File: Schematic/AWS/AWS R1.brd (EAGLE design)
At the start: 50 x 70 mm, 24 parts, among them U1 SN754410_NE_16

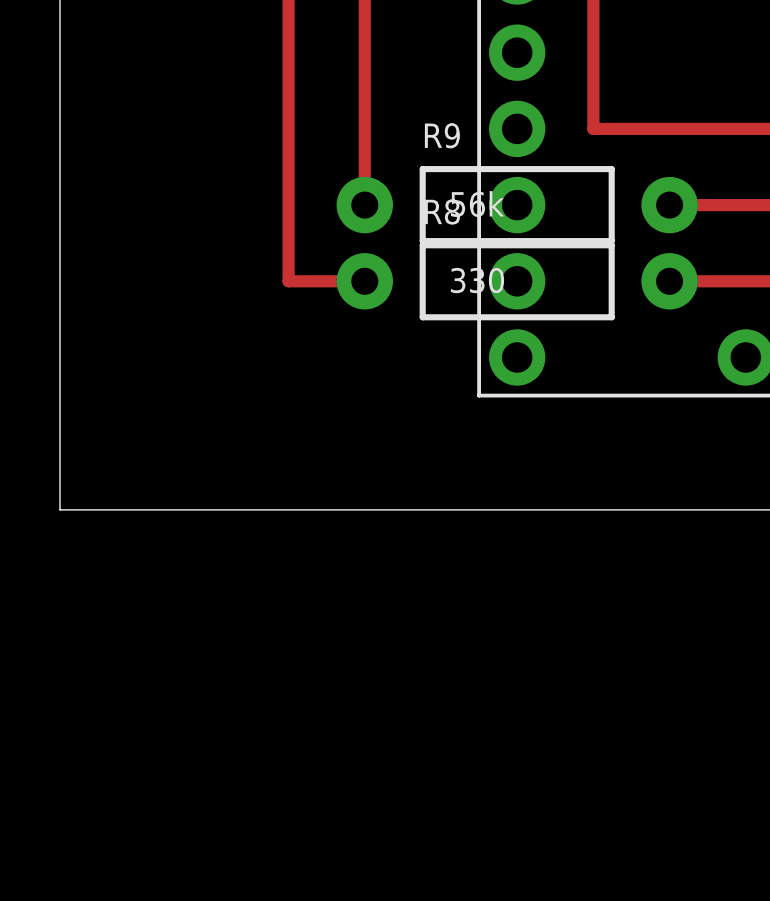
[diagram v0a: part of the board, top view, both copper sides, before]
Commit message: Moved outside
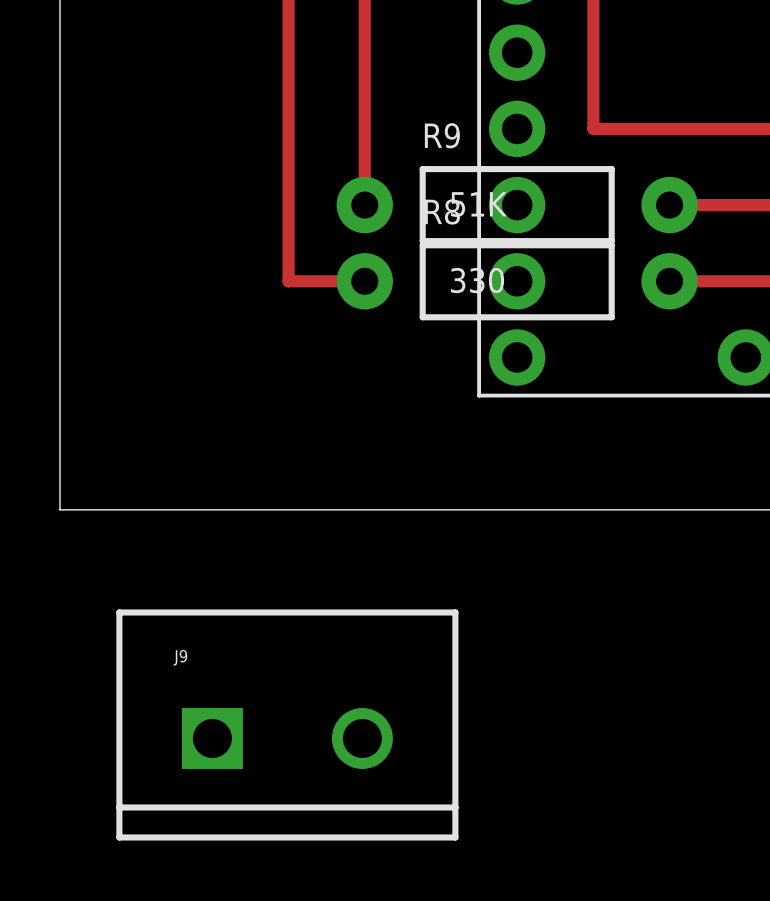
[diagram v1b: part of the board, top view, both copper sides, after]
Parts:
- added J9: (no value), SparkFun-Connectors:SCREWTERMINAL-5MM-2
- R9: value 56k -> 51K
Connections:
- new net D0: J9.2, U$1.D0
- net A6: now also J9.1
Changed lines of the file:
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@@
 <element name="R7" library="SparkFun-Resistors" package="AXIAL-0.4" value="3.3k" x="33.02" y="12.7" rot="MR0"/>
 <element name="R8" library="SparkFun-Resistors" package="AXIAL-0.4" value="330" x="15.24" y="7.62"/>
-<element name="R9" library="SparkFun-Resistors" package="AXIAL-0.4" value="56k" x="15.24" y="10.16"/>
+<element name="R9" library="SparkFun-Resistors" package="AXIAL-0.4" value="51K" x="15.24" y="10.16"/>
 <element name="U$1" library="MoteinoR4Mod" package="MOTEINTO_R4_SQ" value="MOTEINO_R4_MODULEUSING_SQ_POST_PINS" x="25.4" y="20.32" rot="R270"/>
 <element name="U1" library="SN754410" package="NE16" value="SN754410_NE_16" x="27.94" y="38.1">
@@
 </element>
 <element name="U$3" library="GeekAmmo" package="MC331XX" value="PTC" x="38.1" y="53.34" rot="R90"/>
+<element name="J9" library="SparkFun-Connectors" package="SCREWTERMINAL-5MM-2" value="" x="5.08" y="-7.62">
+<attribute name="STOREFRONT_ID" value="PRT-08432" x="5.08" y="-7.62" size="1.778" layer="27" display="off"/>
+</element>
 </elements>
 <signals>
@@
 <contactref element="R9" pad="P$1"/>
 <contactref element="J8" pad="1"/>
-<wire x1="35.56" y1="20.32" x2="7.62" y2="27.94" width="0" layer="19" extent="1-1"/>
 <wire x1="10.16" y1="10.16" x2="10.16" y2="27.94" width="0.4064" layer="1"/>
 <wire x1="10.16" y1="27.94" x2="7.62" y2="27.94" width="0.4064" layer="1"/>
+<contactref element="J9" pad="1"/>
+<wire x1="10.16" y1="27.94" x2="35.56" y2="20.32" width="0" layer="19" extent="1-1"/>
+<wire x1="5.08" y1="-7.62" x2="10.16" y2="10.16" width="0" layer="19" extent="1-1"/>
 </signal>
 <signal name="A2">
@@
 <wire x1="45.72" y1="58.57" x2="45.72" y2="58.42" width="0.4064" layer="1"/>
 </signal>
+<signal name="D0">
+<contactref element="J9" pad="2"/>
+<contactref element="U$1" pad="D0"/>
+<wire x1="10.08" y1="-7.62" x2="35.56" y2="25.4" width="0" layer="19" extent="1-1"/>
+</signal>
 </signals>
